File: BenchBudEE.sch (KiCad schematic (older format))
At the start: 0 parts

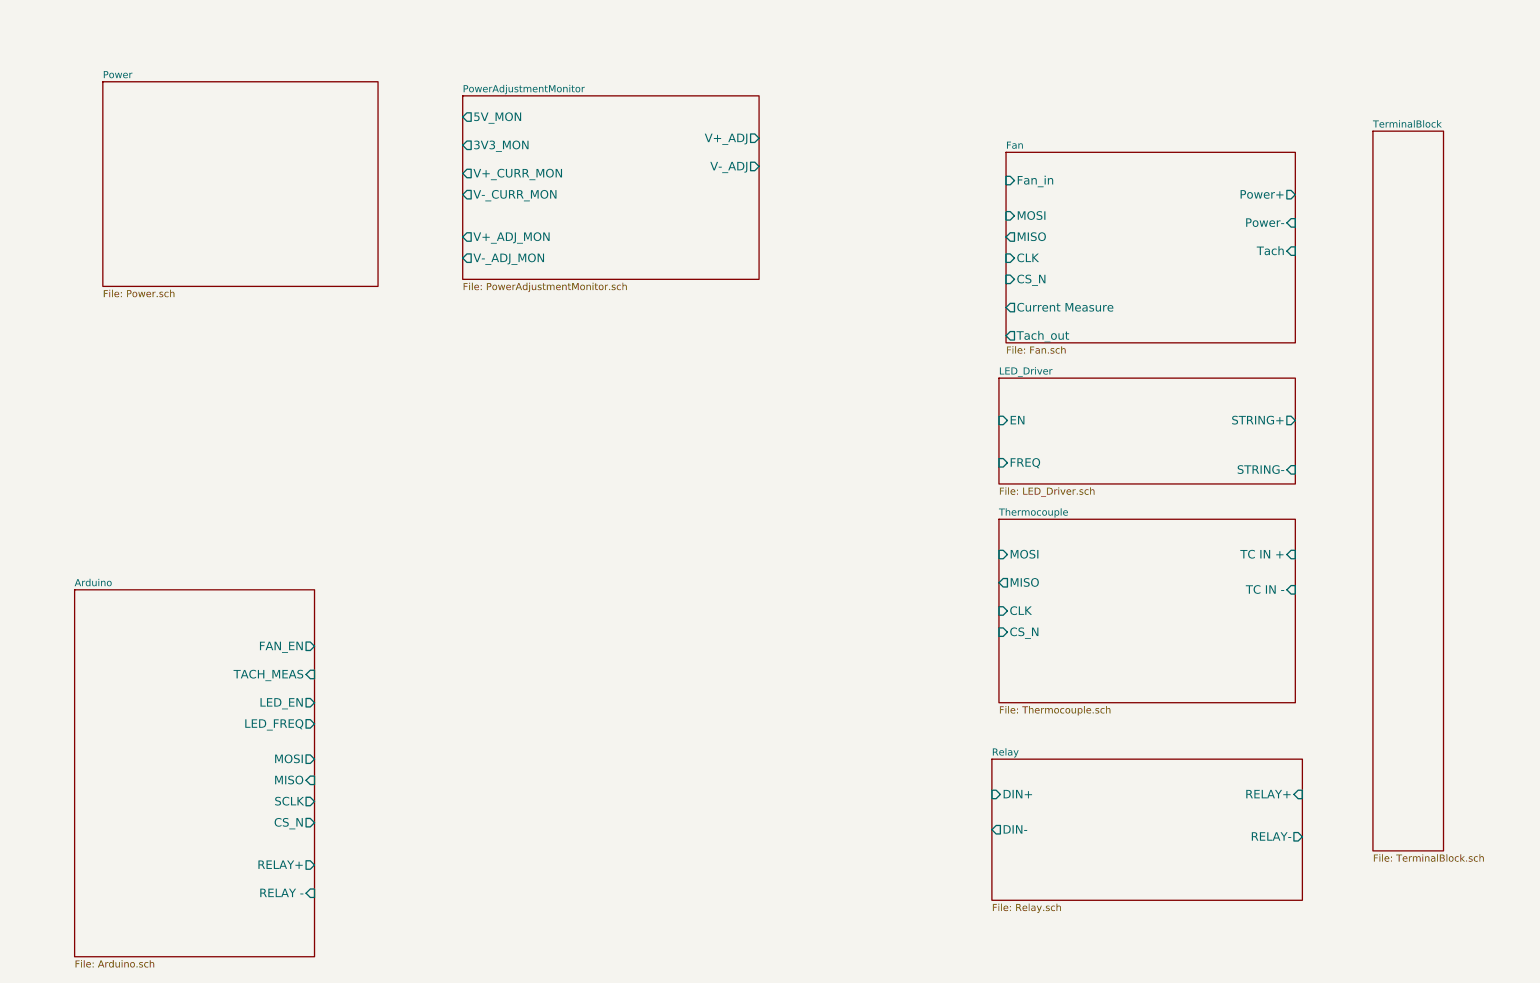
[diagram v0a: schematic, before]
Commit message: Finished Week 3, Unit 10: Revisiting The Current Fan Module
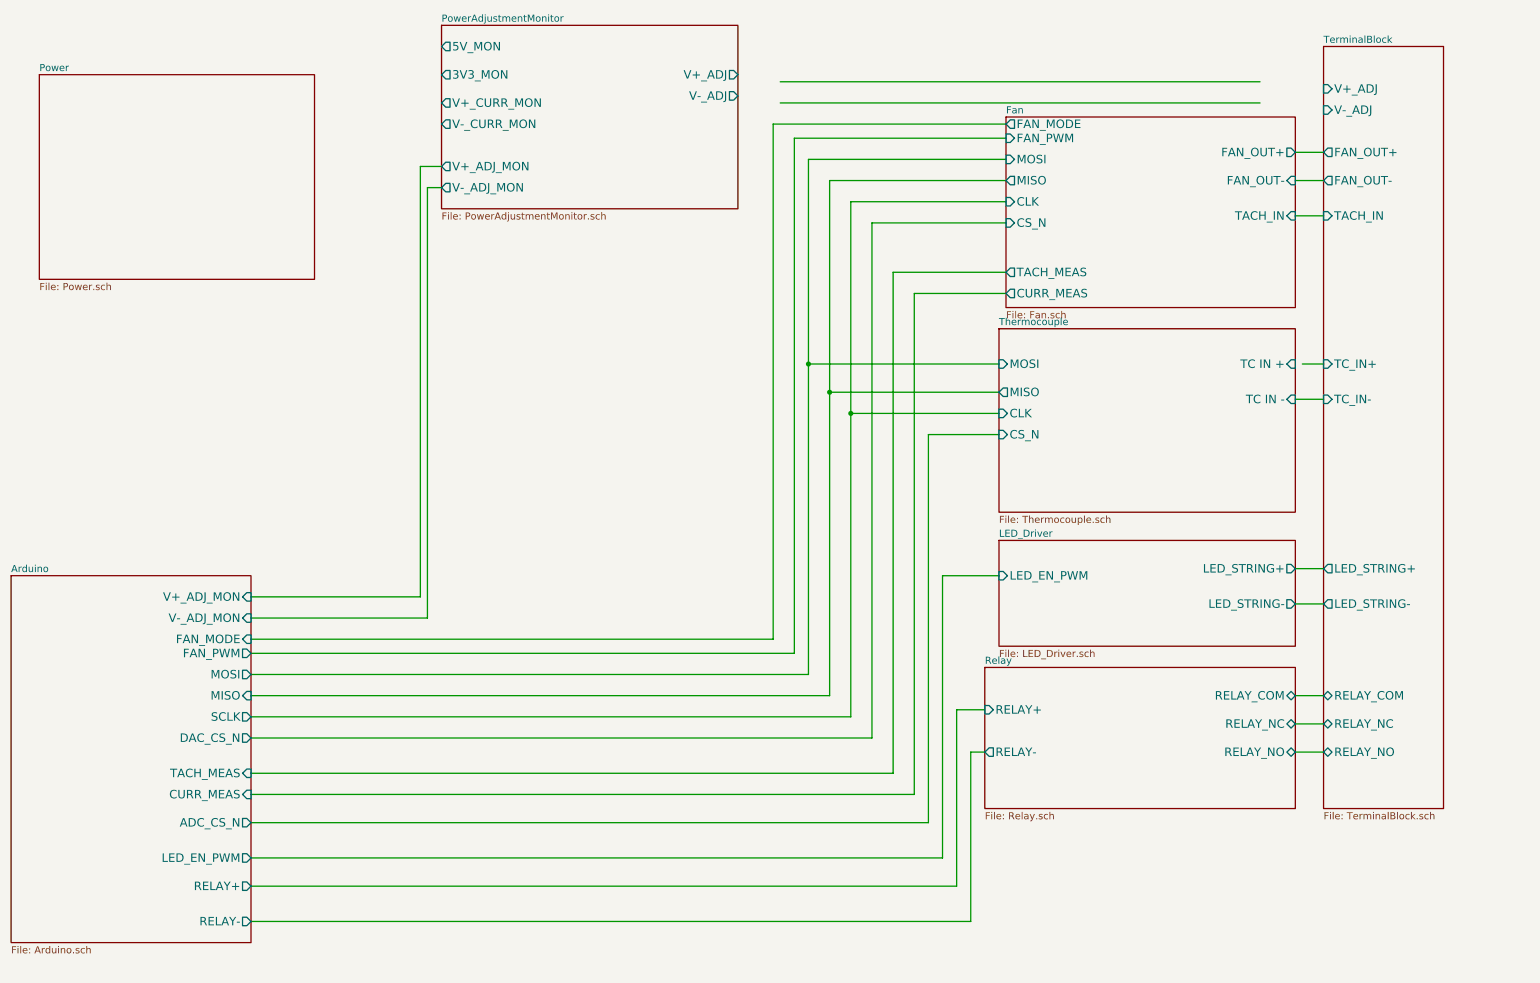
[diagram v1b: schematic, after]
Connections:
- wire segments 0 -> 57
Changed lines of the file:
@@
 LIBS:valves
 LIBS:BenchBudEE
+LIBS:arduino_shieldsNCL
 LIBS:BenchBudEE-cache
 EELAYER 27 0
@@
 Sheet 1 9
 Title ""
-Date "6 feb 2014"
+Date "7 feb 2014"
 Rev ""
 Comp ""
@@
 $EndDescr
 $Sheet
-S 1450 4800 1700 2600
+S 8000 2950 2100 1300
+U 52ED0C08
+F0 "Thermocouple" 50
+F1 "Thermocouple.sch" 50
+F2 "TC IN +" I R 10100 3200 60
+F3 "TC IN -" I R 10100 3450 60
+F4 "MOSI" I L 8000 3200 60
+F5 "MISO" O L 8000 3400 60
+F6 "CLK" I L 8000 3550 60
+F7 "CS_N" I L 8000 3700 60
+$EndSheet
+$Sheet
+S 7900 5350 2200 1000
+U 52ED0C34
+F0 "Relay" 50
+F1 "Relay.sch" 50
+F2 "RELAY_NC" B R 10100 5750 60
+F3 "RELAY_NO" B R 10100 5950 60
+F4 "RELAY_COM" B R 10100 5550 60
+F5 "RELAY+" I L 7900 5650 60
+F6 "RELAY-" O L 7900 5950 60
+$EndSheet
+$Sheet
+S 1200 1150 1950 1450
+U 52ED0C78
+F0 "Power" 50
+F1 "Power.sch" 50
+$EndSheet
+$Sheet
+S 8000 4450 2100 750
+U 52ED0CB4
+F0 "LED_Driver" 50
+F1 "LED_Driver.sch" 50
+F2 "LED_EN_PWM" I L 8000 4700 60
+F3 "LED_STRING+" O R 10100 4650 60
+F4 "LED_STRING-" O R 10100 4900 60
+$EndSheet
+$Sheet
+S 10300 950  850  5400
+U 52ED0D18
+F0 "TerminalBlock" 50
+F1 "TerminalBlock.sch" 50
+F2 "V+_ADJ" I L 10300 1250 60
+F3 "V-_ADJ" I L 10300 1400 60
+F4 "FAN_OUT+" O L 10300 1700 60
+F5 "FAN_OUT-" O L 10300 1900 60
+F6 "TACH_IN" I L 10300 2150 60
+F7 "LED_STRING+" O L 10300 4650 60
+F8 "LED_STRING-" O L 10300 4900 60
+F9 "TC_IN+" I L 10300 3200 60
+F10 "TC_IN-" I L 10300 3450 60
+F11 "RELAY_COM" B L 10300 5550 60
+F12 "RELAY_NO" B L 10300 5950 60
+F13 "RELAY_NC" B L 10300 5750 60
+$EndSheet
+$Sheet
+S 4050 800  2100 1300
+U 52F22A27
+F0 "PowerAdjustmentMonitor" 50
+F1 "PowerAdjustmentMonitor.sch" 50
+F2 "V+_ADJ" O R 6150 1150 60
+F3 "V-_ADJ" O R 6150 1300 60
+F4 "3V3_MON" O L 4050 1150 60
+F5 "5V_MON" O L 4050 950 60
+F6 "V+_ADJ_MON" O L 4050 1800 60
+F7 "V-_ADJ_MON" O L 4050 1950 60
+F8 "V+_CURR_MON" O L 4050 1350 60
+F9 "V-_CURR_MON" O L 4050 1500 60
+$EndSheet
+Wire Wire Line
+	6450 1200 9850 1200
+Wire Wire Line
+	6450 1350 9850 1350
+Wire Wire Line
+	10100 1700 10300 1700
+Wire Wire Line
+	10100 1900 10300 1900
+Wire Wire Line
+	10100 2150 10300 2150
+Wire Wire Line
+	10100 5550 10300 5550
+Wire Wire Line
+	10100 5750 10300 5750
+Wire Wire Line
+	10100 5950 10300 5950
+Wire Wire Line
+	3900 4850 2700 4850
+Wire Wire Line
+	3900 1800 3900 4850
+Wire Wire Line
+	3900 1800 4050 1800
+Wire Wire Line
+	2700 5000 3950 5000
+Wire Wire Line
+	10150 3200 10300 3200
+Wire Wire Line
+	10100 3450 10300 3450
+Wire Wire Line
+	10100 4650 10300 4650
+Wire Wire Line
+	10100 4900 10300 4900
+$Sheet
+S 1000 4700 1700 2600
 U 52ED0B6E
 F0 "Arduino" 50
 F1 "Arduino.sch" 50
-F2 "RELAY+" O R 3150 6750 60
-F3 "RELAY -" I R 3150 6950 60
-F4 "MOSI" O R 3150 6000 60
-F5 "MISO" I R 3150 6150 60
-F6 "SCLK" O R 3150 6300 60
-F7 "CS_N" O R 3150 6450 60
-F8 "LED_EN" O R 3150 5600 60
-F9 "LED_FREQ" O R 3150 5750 60
-F10 "FAN_EN" O R 3150 5200 60
-F11 "TACH_MEAS" I R 3150 5400 60
-$EndSheet
-$Sheet
-S 8000 4300 2100 1300
-U 52ED0C08
-F0 "Thermocouple" 50
-F1 "Thermocouple.sch" 50
-F2 "TC IN +" I R 10100 4550 60
-F3 "TC IN -" I R 10100 4800 60
-F4 "MOSI" I L 8000 4550 60
-F5 "MISO" O L 8000 4750 60
-F6 "CLK" I L 8000 4950 60
-F7 "CS_N" I L 8000 5100 60
-$EndSheet
-$Sheet
-S 7950 6000 2200 1000
-U 52ED0C34
-F0 "Relay" 50
-F1 "Relay.sch" 50
-F2 "DIN+" I L 7950 6250 60
-F3 "DIN-" O L 7950 6500 60
-F4 "RELAY+" I R 10150 6250 60
-F5 "RELAY-" O R 10150 6550 60
-$EndSheet
-$Sheet
-S 1650 1200 1950 1450
-U 52ED0C78
-F0 "Power" 50
-F1 "Power.sch" 50
-$EndSheet
-$Sheet
-S 8000 3300 2100 750
-U 52ED0CB4
-F0 "LED_Driver" 50
-F1 "LED_Driver.sch" 50
-F2 "EN" I L 8000 3600 60
-F3 "FREQ" I L 8000 3900 60
-F4 "STRING+" O R 10100 3600 60
-F5 "STRING-" I R 10100 3950 60
-$EndSheet
-$Sheet
-S 10650 1550 500  5100
-U 52ED0D18
-F0 "TerminalBlock" 50
-F1 "TerminalBlock.sch" 50
-$EndSheet
-$Sheet
-S 8050 1700 2050 1350
+F2 "RELAY+" O R 2700 6900 60
+F3 "MOSI" O R 2700 5400 60
+F4 "MISO" I R 2700 5550 60
+F5 "SCLK" O R 2700 5700 60
+F6 "TACH_MEAS" I R 2700 6100 60
+F7 "RELAY-" O R 2700 7150 60
+F8 "CURR_MEAS" I R 2700 6250 60
+F9 "V+_ADJ_MON" I R 2700 4850 60
+F10 "V-_ADJ_MON" I R 2700 5000 60
+F11 "LED_EN_PWM" O R 2700 6700 60
+F12 "DAC_CS_N" O R 2700 5850 60
+F13 "ADC_CS_N" O R 2700 6450 60
+F14 "FAN_PWM" O R 2700 5250 60
+F15 "FAN_MODE" I R 2700 5150 60
+$EndSheet
+Wire Wire Line
+	2700 5250 6550 5250
+Wire Wire Line
+	6550 5250 6550 1600
+Wire Wire Line
+	6550 1600 8050 1600
+Wire Wire Line
+	6650 5400 2700 5400
+Wire Wire Line
+	6650 1750 6650 5400
+Wire Wire Line
+	6650 1750 8050 1750
+Wire Wire Line
+	6800 5550 2700 5550
+Wire Wire Line
+	6800 1900 6800 5550
+Wire Wire Line
+	6800 1900 8050 1900
+Wire Wire Line
+	6950 5700 2700 5700
+Wire Wire Line
+	6950 2050 6950 5700
+Wire Wire Line
+	6950 2050 8050 2050
+Wire Wire Line
+	2700 5850 7100 5850
+Wire Wire Line
+	7100 5850 7100 2200
+Wire Wire Line
+	7100 2200 8050 2200
+Wire Wire Line
+	8000 3200 6650 3200
+Connection ~ 6650 3200
+Wire Wire Line
+	8000 3400 6800 3400
+Connection ~ 6800 3400
+Wire Wire Line
+	8000 3550 6950 3550
+Connection ~ 6950 3550
+Wire Wire Line
+	2700 6100 7250 6100
+Wire Wire Line
+	7250 6100 7250 2550
+Wire Wire Line
+	7250 2550 8050 2550
+Wire Wire Line
+	2700 6250 7400 6250
+Wire Wire Line
+	7400 6250 7400 2700
+Wire Wire Line
+	7400 2700 8050 2700
+Wire Wire Line
+	2700 6450 7500 6450
+Wire Wire Line
+	7500 6450 7500 3700
+Wire Wire Line
+	7500 3700 8000 3700
+Wire Wire Line
+	2700 6700 7600 6700
+Wire Wire Line
+	7600 6700 7600 4700
+Wire Wire Line
+	7600 4700 8000 4700
+Wire Wire Line
+	2700 6900 7700 6900
+Wire Wire Line
+	7700 6900 7700 5650
+Wire Wire Line
+	7700 5650 7900 5650
+Wire Wire Line
+	2700 7150 7800 7150
+Wire Wire Line
+	7800 7150 7800 5950
+Wire Wire Line
+	7800 5950 7900 5950
+Wire Wire Line
+	3950 5000 3950 1950
+Wire Wire Line
+	3950 1950 4050 1950
+$Sheet
+S 8050 1450 2050 1350
 U 52ED0CE0
 F0 "Fan" 50
 F1 "Fan.sch" 50
-F2 "Power+" O R 10100 2000 60
-F3 "Power-" I R 10100 2200 60
-F4 "Tach" I R 10100 2400 60
-F5 "Tach_out" O L 8050 3000 60
-F6 "Fan_in" I L 8050 1900 60
-F7 "Current Measure" O L 8050 2800 60
-F8 "MOSI" I L 8050 2150 60
-F9 "MISO" O L 8050 2300 60
-F10 "CLK" I L 8050 2450 60
-F11 "CS_N" I L 8050 2600 60
-$EndSheet
-$Sheet
-S 4200 1300 2100 1300
-U 52F22A27
-F0 "PowerAdjustmentMonitor" 50
-F1 "PowerAdjustmentMonitor.sch" 50
-F2 "V+_ADJ" O R 6300 1600 60
-F3 "V-_ADJ" O R 6300 1800 60
-F4 "3V3_MON" O L 4200 1650 60
-F5 "5V_MON" O L 4200 1450 60
-F6 "V+_ADJ_MON" O L 4200 2300 60
-F7 "V-_ADJ_MON" O L 4200 2450 60
-F8 "V+_CURR_MON" O L 4200 1850 60
-F9 "V-_CURR_MON" O L 4200 2000 60
-$EndSheet
+F2 "MOSI" I L 8050 1750 60
+F3 "MISO" O L 8050 1900 60
+F4 "CLK" I L 8050 2050 60
+F5 "CS_N" I L 8050 2200 60
+F6 "FAN_OUT+" O R 10100 1700 60
+F7 "FAN_OUT-" I R 10100 1900 60
+F8 "TACH_IN" I R 10100 2150 60
+F9 "TACH_MEAS" O L 8050 2550 60
+F10 "CURR_MEAS" O L 8050 2700 60
+F11 "FAN_PWM" I L 8050 1600 60
+F12 "FAN_MODE" O L 8050 1500 60
+$EndSheet
+Wire Wire Line
+	8050 1500 6400 1500
+Wire Wire Line
+	6400 1500 6400 5150
+Wire Wire Line
+	6400 5150 2700 5150
 $EndSCHEMATC
